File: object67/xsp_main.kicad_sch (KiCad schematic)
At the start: 0 parts

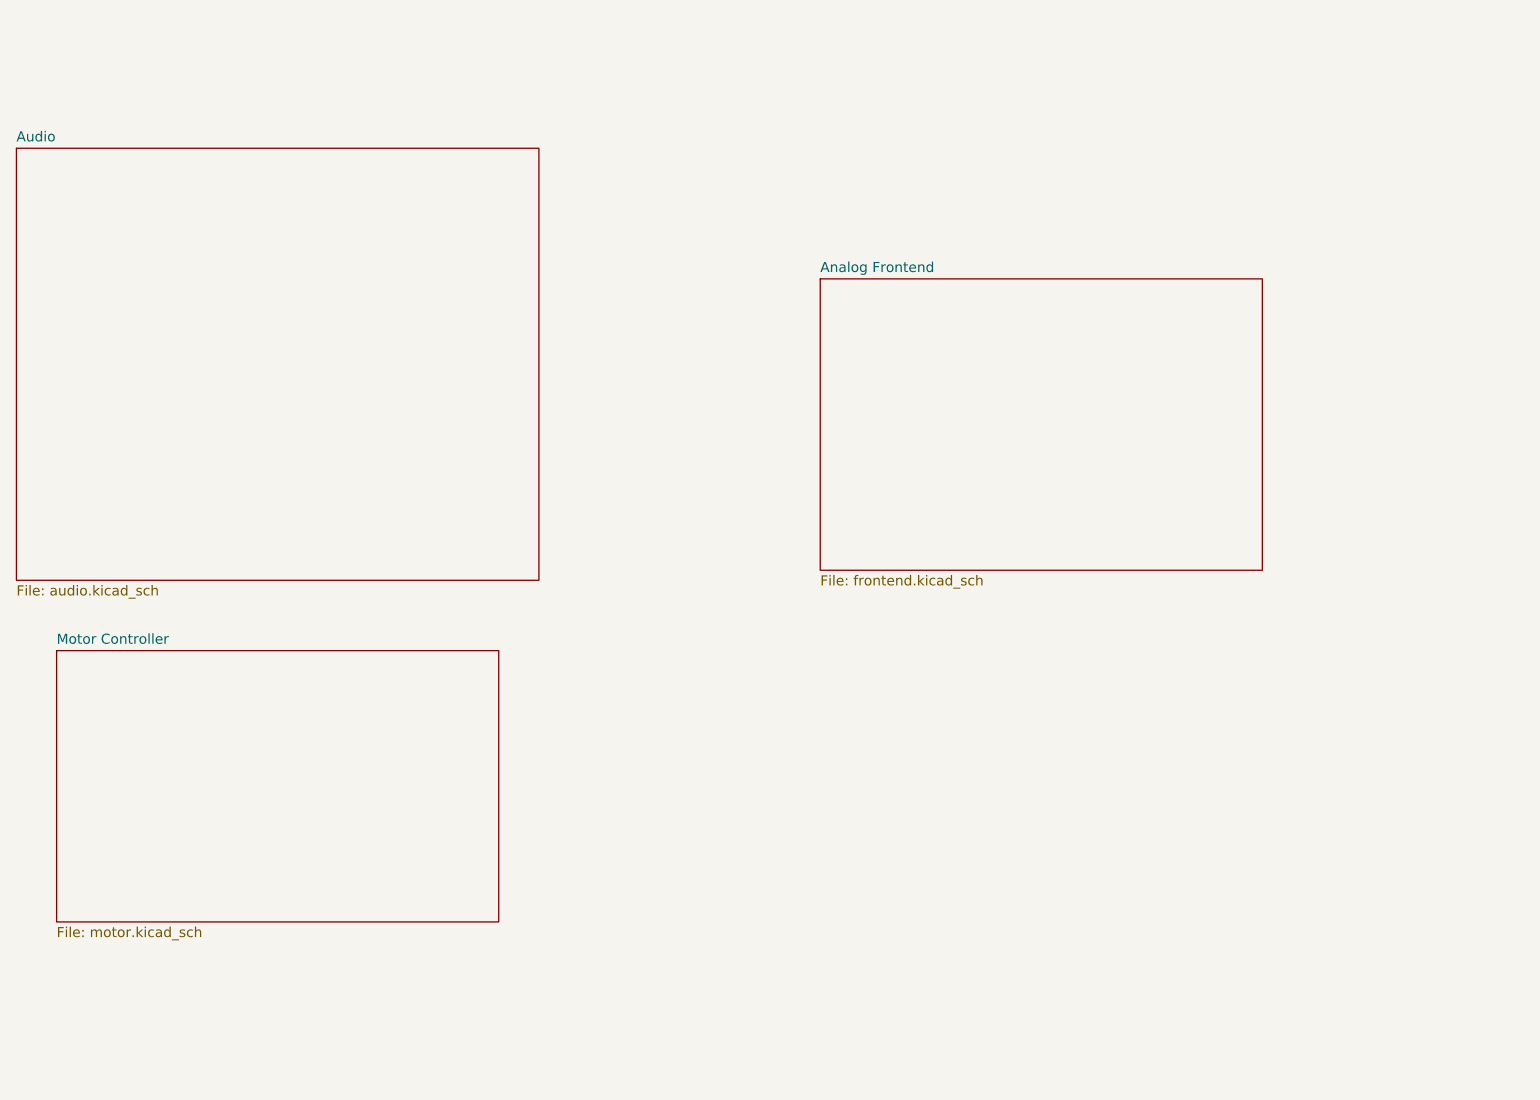
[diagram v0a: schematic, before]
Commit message: ????
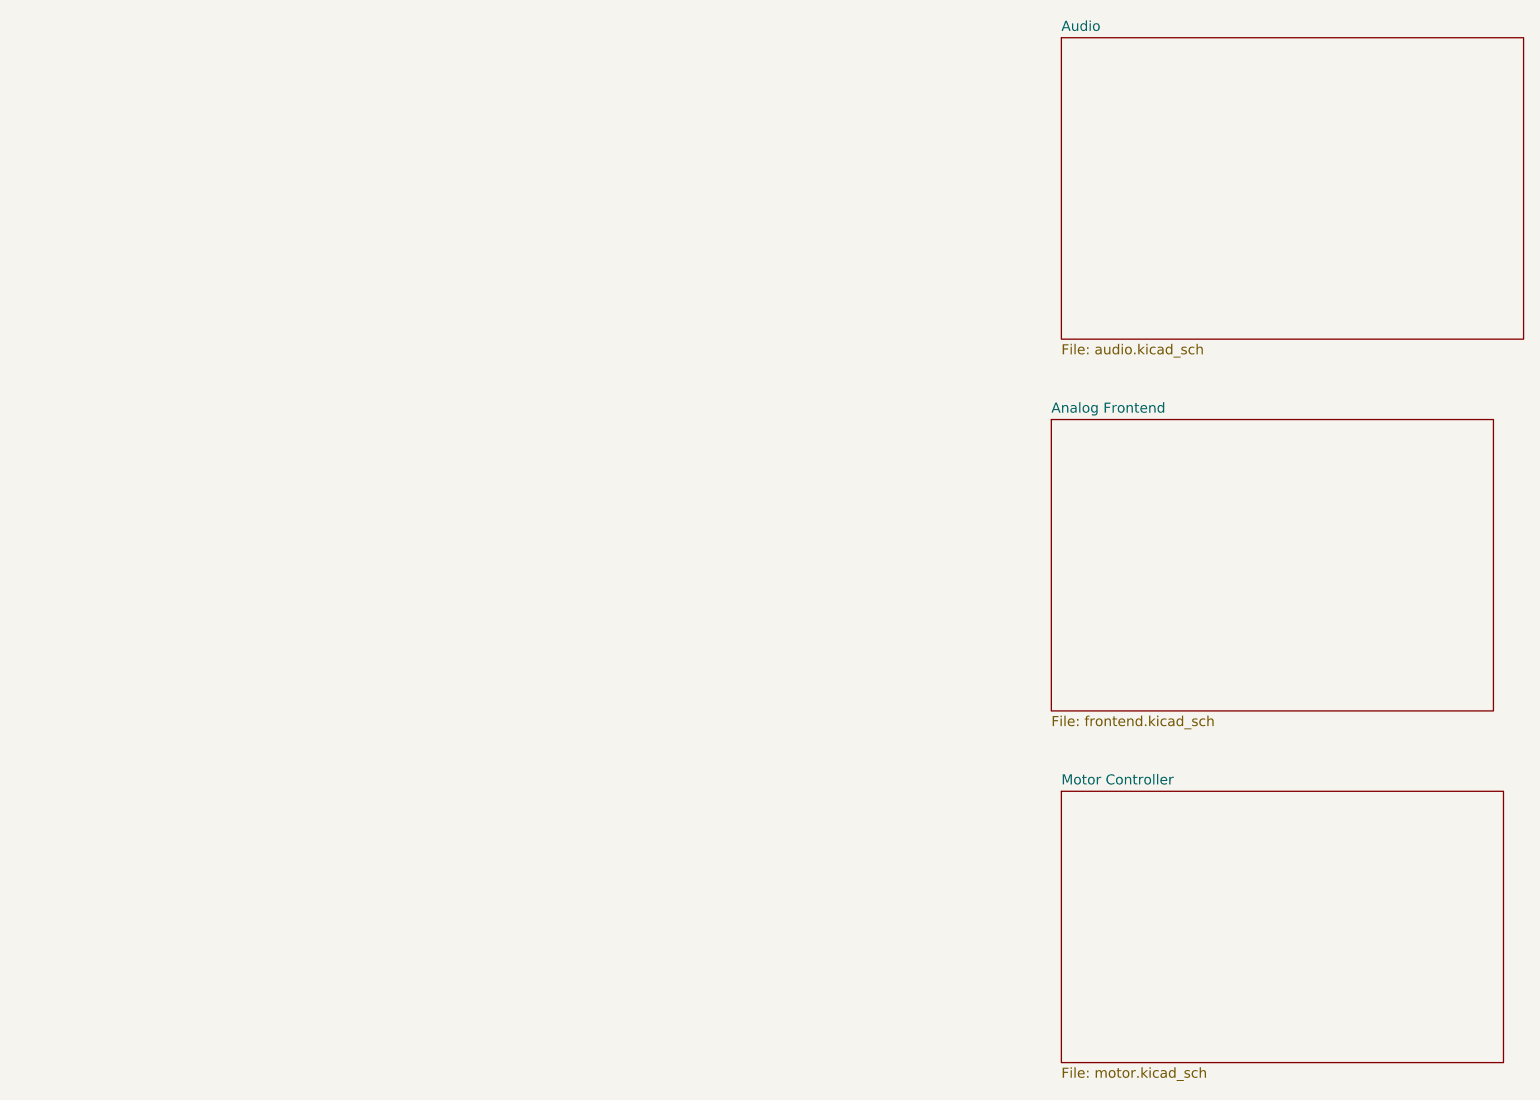
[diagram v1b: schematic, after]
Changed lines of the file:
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@@
 	(paper "A4")
 	(sheet
-		(at 78.74 100.33)
+		(at 205.74 118.11)
 		(size 55.88 34.29)
 		(exclude_from_sim no)
@@
 		)
 		(property "Sheetname" "Motor Controller"
-			(at 78.74 99.6184 0)
+			(at 205.74 117.3984 0)
 			(effects
 				(font
@@
 		)
 		(property "Sheetfile" "motor.kicad_sch"
-			(at 78.74 135.2046 0)
+			(at 205.74 152.9846 0)
 			(effects
 				(font
@@
 	)
 	(sheet
-		(at 175.26 53.34)
+		(at 204.47 71.12)
 		(size 55.88 36.83)
 		(exclude_from_sim no)
@@
 		)
 		(property "Sheetname" "Analog Frontend"
-			(at 175.26 52.6284 0)
+			(at 204.47 70.4084 0)
 			(effects
 				(font
@@
 		)
 		(property "Sheetfile" "frontend.kicad_sch"
-			(at 175.26 90.7546 0)
+			(at 204.47 108.5346 0)
 			(effects
 				(font
@@
 	)
 	(sheet
-		(at 73.66 36.83)
-		(size 66.04 54.61)
+		(at 205.74 22.86)
+		(size 58.42 38.1)
 		(exclude_from_sim no)
 		(in_bom yes)
@@
 		)
 		(property "Sheetname" "Audio"
-			(at 73.66 36.1184 0)
+			(at 205.74 22.1484 0)
 			(effects
 				(font
@@
 		)
 		(property "Sheetfile" "audio.kicad_sch"
-			(at 73.66 92.0246 0)
+			(at 205.74 61.5446 0)
 			(effects
 				(font
